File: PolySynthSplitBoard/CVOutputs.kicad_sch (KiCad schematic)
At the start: 121 parts, among them U301 DAC7578xPW, U302 TL074, U303 TL072, U304 TL074, U305 TL072, U306 TMUX4051, U307 TL074, U308 TMUX4051, U309 TL072, U310 TL074, U311 TL072, U312 TL074, U313 TMUX4051, U314 TMUX4051, U315 TL074, U316 TL074, U317 TL074, U318 TL072, U319 TL072, U320 TL072, U321 TMUX4051, U322 TMUX4051, U323 TMUX4051

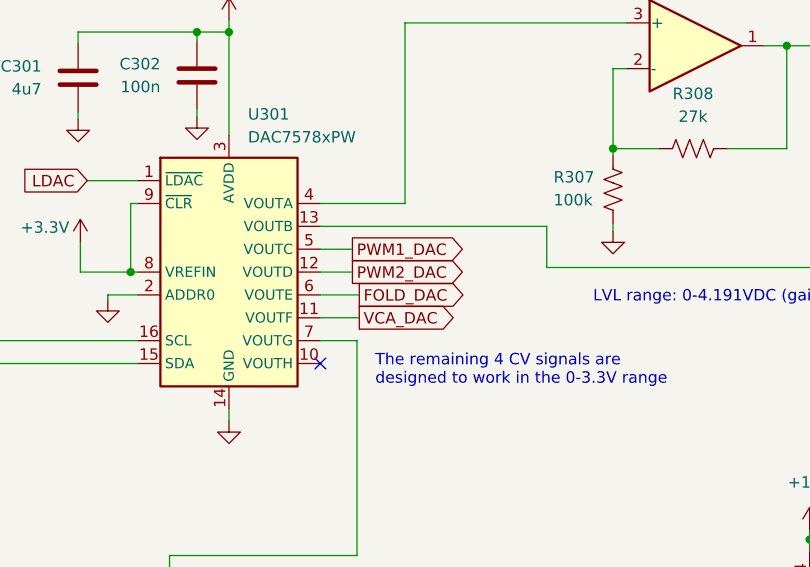
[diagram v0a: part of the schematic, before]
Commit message: lower board
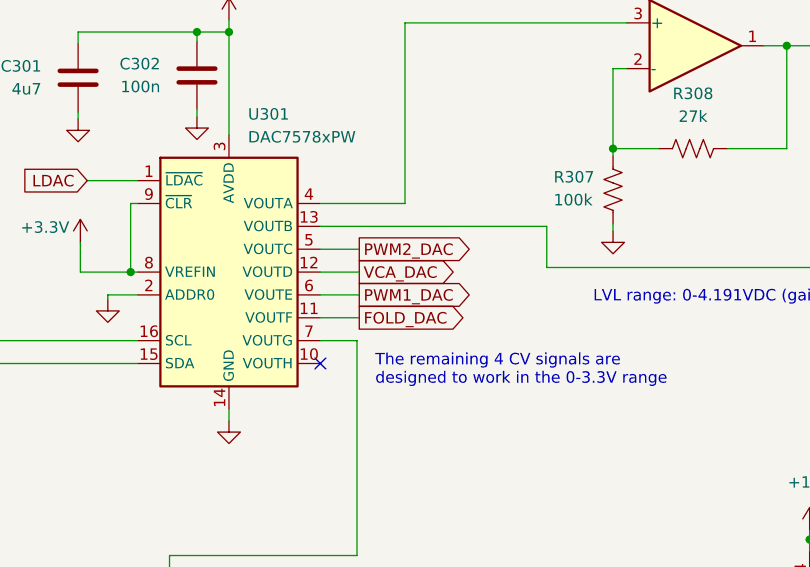
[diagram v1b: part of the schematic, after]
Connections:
- net FOLD_DAC: now also U301.11 (VOUTF); no longer U301.6 (VOUTE)
- net PWM1_DAC: now also U301.6 (VOUTE); no longer U301.5 (VOUTC)
- net PWM2_DAC: now also U301.5 (VOUTC); no longer U301.12 (VOUTD)
- net VCA_DAC: now also U301.12 (VOUTD); no longer U301.11 (VOUTF)
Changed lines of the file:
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@@
 	(wire
 		(pts
-			(xy 76.2 71.628) (xy 79.756 71.628)
+			(xy 76.2 71.628) (xy 80.518 71.628)
 		)
 		(stroke
@@
 	(wire
 		(pts
+			(xy 76.2 69.088) (xy 80.518 69.088)
+		)
+		(stroke
+			(width 0)
+			(type default)
+		)
+	)
+	(wire
+		(pts
 			(xy 432.816 125.984) (xy 432.816 117.094)
 		)
@@
 	(wire
 		(pts
-			(xy 76.2 69.088) (xy 79.756 69.088)
-		)
-		(stroke
-			(width 0)
-			(type default)
-		)
-	)
-	(wire
-		(pts
 			(xy 495.808 176.276) (xy 500.888 176.276)
 		)
@@
 	(global_label "PWM2_DAC"
 		(shape output)
-		(at 79.756 71.628 0)
+		(at 80.518 69.088 0)
 		(fields_autoplaced yes)
 		(effects
@@
 		)
 		(property "Intersheetrefs" "${INTERSHEET_REFS}"
-			(at 92.7197 71.628 0)
+			(at 93.4817 69.088 0)
 			(effects
 				(font
@@
 	(global_label "VCA_DAC"
 		(shape output)
-		(at 80.518 76.708 0)
+		(at 80.518 71.628 0)
 		(fields_autoplaced yes)
 		(effects
@@
 		)
 		(property "Intersheetrefs" "${INTERSHEET_REFS}"
-			(at 91.5466 76.708 0)
+			(at 91.5466 71.628 0)
 			(effects
 				(font
@@
 	(global_label "PWM1_DAC"
 		(shape output)
-		(at 79.756 69.088 0)
+		(at 80.518 74.168 0)
 		(fields_autoplaced yes)
 		(effects
@@
 		)
 		(property "Intersheetrefs" "${INTERSHEET_REFS}"
-			(at 92.7197 69.088 0)
+			(at 93.4817 74.168 0)
 			(effects
 				(font
@@
 	(global_label "FOLD_DAC"
 		(shape output)
-		(at 80.518 74.168 0)
+		(at 80.518 76.708 0)
 		(fields_autoplaced yes)
 		(effects
@@
 		)
 		(property "Intersheetrefs" "${INTERSHEET_REFS}"
-			(at 92.8166 74.168 0)
+			(at 92.8166 76.708 0)
 			(effects
 				(font
